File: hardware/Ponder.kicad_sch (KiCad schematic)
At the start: 128 parts, among them J1 USB_C_Receptacle_USB2.0, J10 2.54 SKT, J11 2.54 HDR, J2 2.54 HDR, J3 2.54 HDR, J4 2.54 HDR, J5 2.54 HDR, J6 2.54 HDR, J7 2.54 HDR, J8 2.54 SKT, J9 1.27 HDR, SW1 434133025816, SW2 434133025816, U1 NCP1117-3.3_SOT223, U2 W25Q64JVXGIQ_TR, U3 RP2350_80QFN, U4 18012115411H, U5 18012115411H, U6 18012115411H, U7 18012115411H, U8 18012115411H, U9 18012115411H, X1 ABM8-272-T3

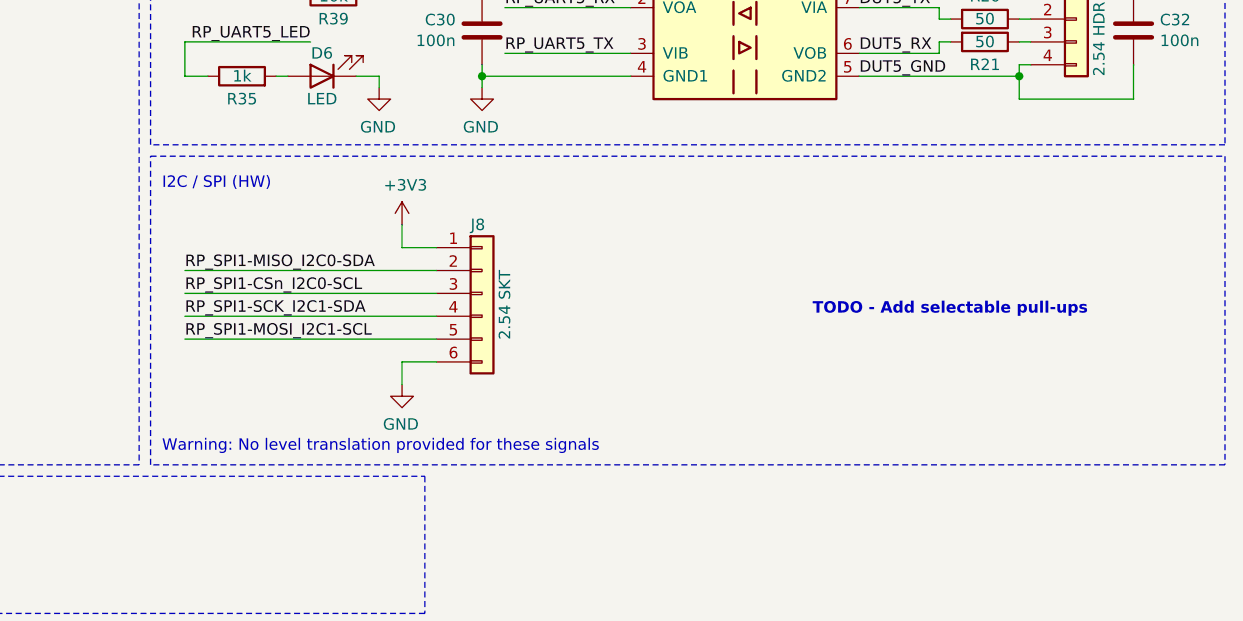
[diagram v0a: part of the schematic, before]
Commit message: Silk tittivating
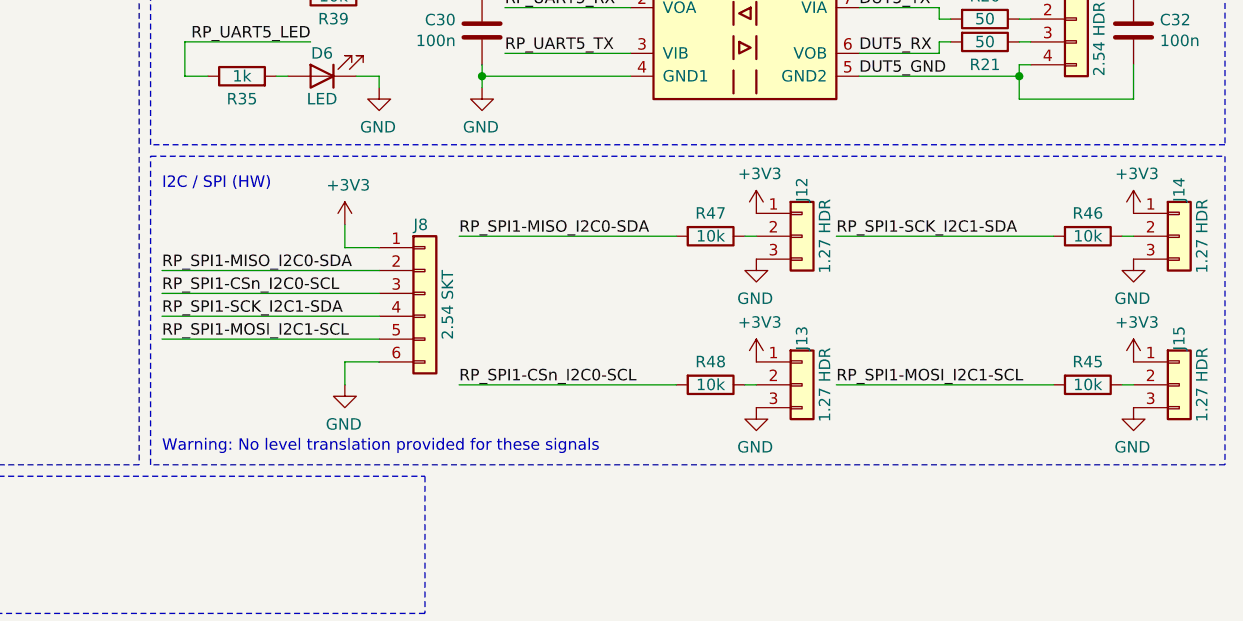
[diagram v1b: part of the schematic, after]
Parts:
- added J12, J13, J14, J15: 1.27 HDR, Connector_PinHeader_1.27mm:PinHeader_1x03_P1.27mm_Vertical, symbol Connector_Generic:Conn_01x03
- added R45, R46, R47, R48: 10k, Resistor_SMD:R_0402_1005Metric, symbol Device:R
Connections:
- net +3V3: now also J12.1 (Pin_1), J13.1 (Pin_1), J14.1 (Pin_1), J15.1 (Pin_1)
- net GND: now also J12.3 (Pin_3), J13.3 (Pin_3), J14.3 (Pin_3), J15.3 (Pin_3)
- net RP_SPI1-CSn_I2C0-SCL: now also R48.2
- net RP_SPI1-MISO_I2C0-SDA: now also R47.2
- net RP_SPI1-MOSI_I2C1-SCL: now also R45.2
- net RP_SPI1-SCK_I2C1-SDA: now also R46.2
- new net: J12.2 (Pin_2), R47.1
- new net: J15.2 (Pin_2), R45.1
- new net: J14.2 (Pin_2), R46.1
- new net: J13.2 (Pin_2), R48.1
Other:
- note removed: "TODO - Add selectable pull-ups"
- moved on the sheet: J8
